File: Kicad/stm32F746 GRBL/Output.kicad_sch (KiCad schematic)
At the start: 23 parts, among them J16 Output, J17 PWM-1, J18 PWM-2, J19 PWM-3, J20 PWM-4, Q1 BSS138, Q2 BSS138, Q3 BSS138, Q4 BSS138, U12 ULN2803A, U13 TS921, U14 TLP185, U4 MCP23017_SS

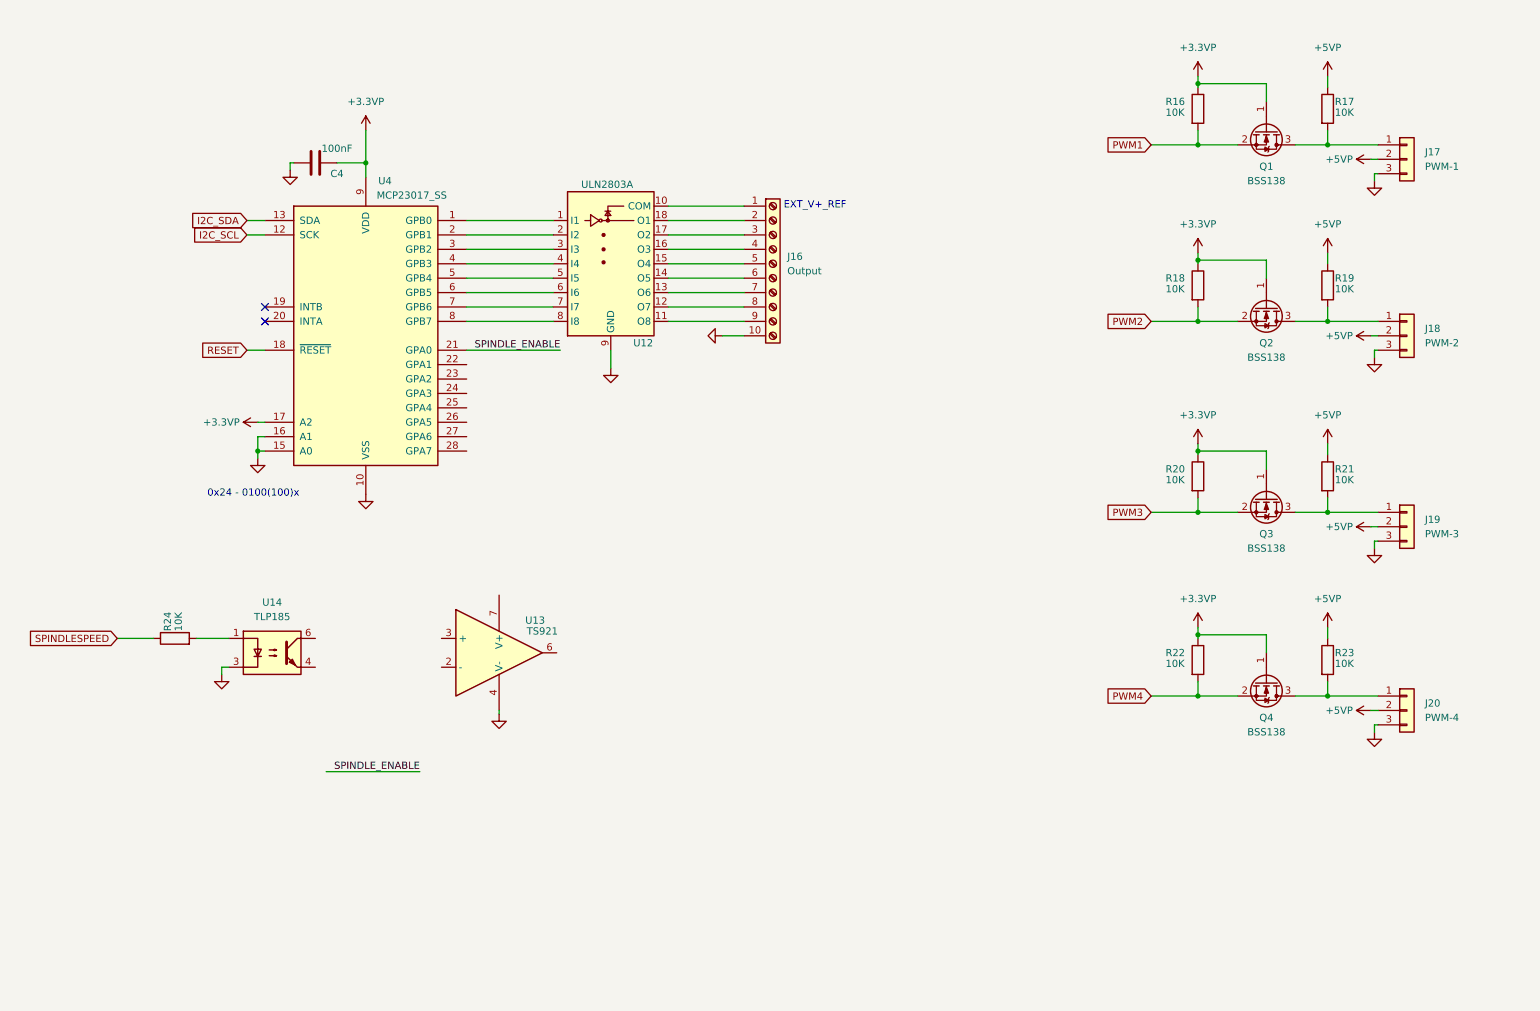
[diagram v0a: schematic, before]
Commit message: wip kicad
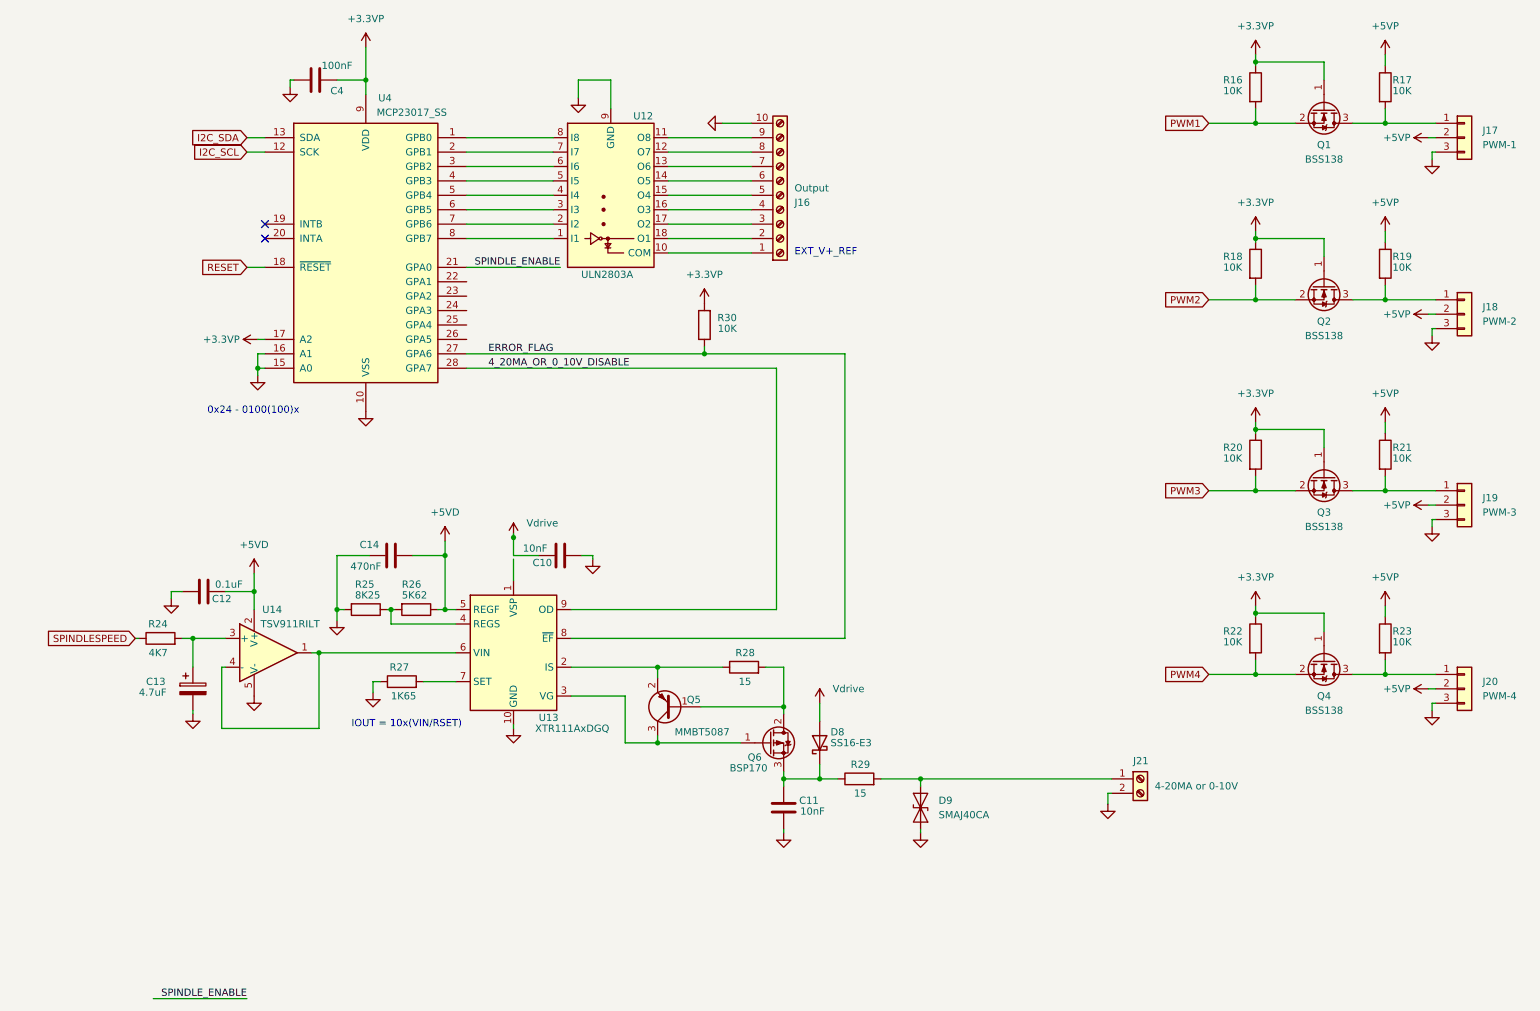
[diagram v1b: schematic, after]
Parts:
- removed U13: TS921, Package_SO:TSSOP-8_4.4x3mm_P0.65mm, symbol stm32F746 GRBL:TS921
- removed U14: TLP185, Package_SO:SOIC-4_4.55x3.7mm_P2.54mm, symbol Isolator:TLP185
- added C10, C11: 10nF, Capacitor_SMD:C_0805_2012Metric, symbol Device:C
- added C12: 0.1uF, Capacitor_SMD:C_0805_2012Metric, symbol Device:C
- added C13: 4.7uF, Capacitor_SMD:C_0805_2012Metric, symbol Device:C_Polarized
- added C14: 470nF, Capacitor_SMD:C_0805_2012Metric, symbol Device:C
- added D8: SS16-E3, symbol Device:D_Schottky
- added D9: SMAJ40CA, Diode_SMD:D_SMA, symbol Diode:SMAJ40CA
- added J21: 4-20MA or 0-10V, TerminalBlock_TE-Connectivity:TerminalBlock_TE_282834-2_1x02_P2.54mm_Horizontal, symbol Connector:Screw_Terminal_01x02
- added Q5: MMBT5087, Package_TO_SOT_SMD:SOT-23, symbol Transistor_BJT:MMBT3906
- added Q6: BSP170, Package_TO_SOT_SMD:SOT-223-3_TabPin2, symbol Transistor_FET:ZXMP4A16G
- added R25: 8K25, Resistor_SMD:R_0805_2012Metric_Pad1.20x1.40mm_HandSolder, symbol Device:R
- added R26: 5K62, Resistor_SMD:R_0805_2012Metric_Pad1.20x1.40mm_HandSolder, symbol Device:R
- added R27: 1K65, Resistor_SMD:R_0805_2012Metric_Pad1.20x1.40mm_HandSolder, symbol Device:R
- added R28, R29: 15, Resistor_SMD:R_0805_2012Metric_Pad1.20x1.40mm_HandSolder, symbol Device:R
- added R30: 10K, Resistor_SMD:R_0805_2012Metric_Pad1.20x1.40mm_HandSolder, symbol Device:R
- added U13: XTR111AxDGQ, Package_SO:MSOP-10-1EP_3x3mm_P0.5mm_EP2.2x3.1mm_Mask1.83x1.89mm_ThermalVias, symbol Interface_CurrentLoop:XTR111AxDGQ
- added U14: TSV911RILT, Package_TO_SOT_SMD:SOT-23-5, symbol Amplifier_Operational:TSV911RILT
- R24: value 10K -> 4K7
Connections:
- net +3.3VP: now also R30.2
- net GND: now also C10.2, C11.2, C12.2, C13.2, C14.1, D9.1 (A1), J21.2 (Pin_2), R25.2, R27.1, U13.10 (GND), U13.11 (GND), U14.5 (V-)
- net at U4.1 (GPB0): now also U12.8 (I8); no longer U12.1 (I1)
- net at U4.2 (GPB1): now also U12.7 (I7); no longer U12.2 (I2)
- net at U4.3 (GPB2): now also U12.6 (I6); no longer U12.3 (I3)
- net at U4.4 (GPB3): now also U12.5 (I5); no longer U12.4 (I4)
- net at U4.5 (GPB4): now also U12.4 (I4); no longer U12.5 (I5)
- net at U4.6 (GPB5): now also U12.3 (I3); no longer U12.6 (I6)
- net at U4.7 (GPB6): now also U12.2 (I2); no longer U12.7 (I7)
- net at U4.8 (GPB7): now also U12.1 (I1); no longer U12.8 (I8)
- net at R24.2: now also C13.1, U14.3 (+)
- net ERROR_FLAG: now reaches U4.27 (GPA6)
- net ERROR_FLAG: now also R30.1, U13.8 (~{EF})
- net 4_20MA_OR_0_10V_DISABLE: now reaches U4.28 (GPA7)
- net 4_20MA_OR_0_10V_DISABLE: now also U13.9 (OD)
- new net: Q5.3 (C), Q6.1 (G), U13.3 (VG)
- new net: Q5.1 (B), Q6.2 (D), R28.2
- new net: C11.1, D8.1 (K), Q6.3 (S), R29.1
- new net: R25.1, R26.2, U13.4 (REGS)
- new net: U13.6 (VIN), U14.1, U14.4 (-)
- new net: Q5.2 (E), R28.1, U13.2 (IS)
- new net: R27.2, U13.7 (SET)
- new net: D9.2 (A2), J21.1 (Pin_1), R29.2
- new net +5VD: C12.1, C14.2, R26.1, U13.5 (REGF), U14.2 (V+)
- new net Vdrive: C10.1, D8.2 (A)
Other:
- note added: "IOUT = 10x(VIN/RSET)"
- moved on the sheet: C4, J17, J18, J19, J20, Q1, Q2, Q3, Q4, R16, R17, R18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
